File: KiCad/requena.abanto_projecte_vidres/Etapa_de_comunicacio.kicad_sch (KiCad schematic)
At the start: 13 parts, among them J1 DE9_Pins, J2 DE9_Pins, U1 MAX232, U3 TJA1051TK-3

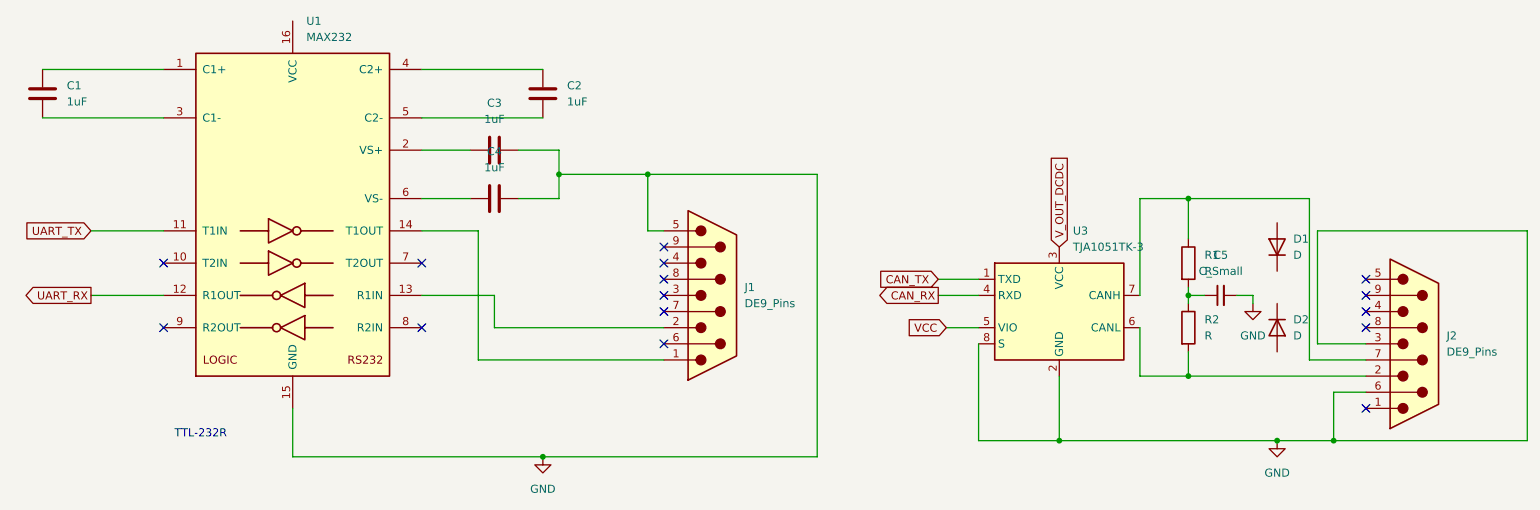
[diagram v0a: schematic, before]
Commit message: arreglos :)
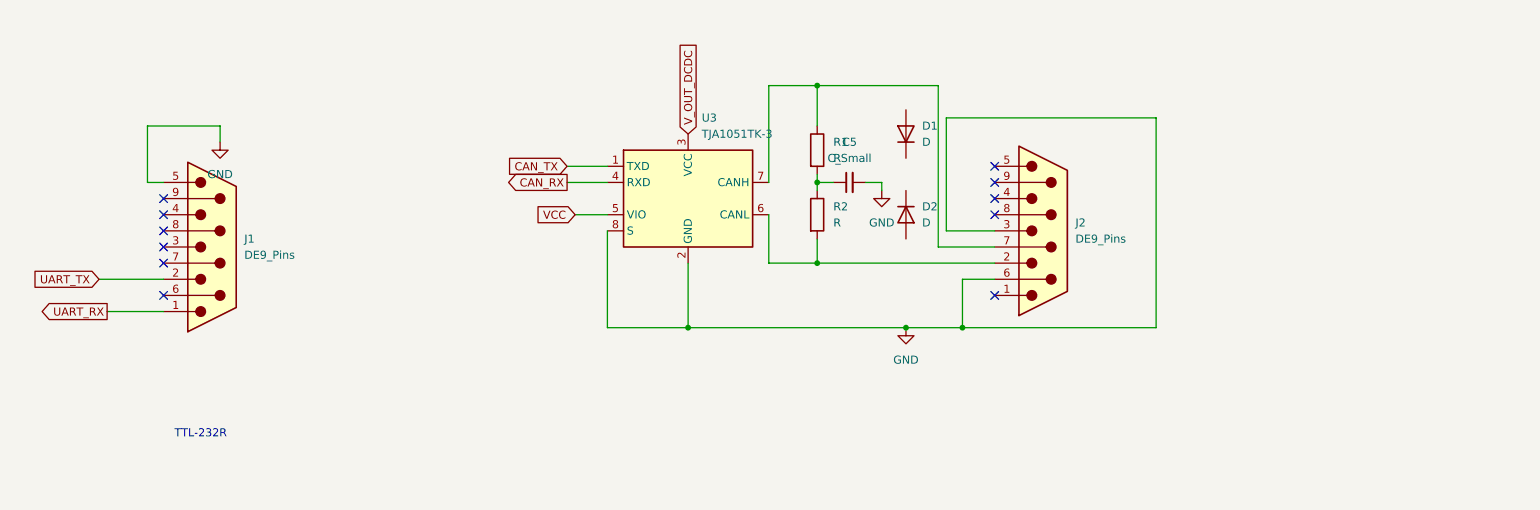
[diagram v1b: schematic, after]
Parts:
- removed C1, C2, C3, C4: 1uF, symbol Device:C
- removed U1: MAX232, symbol Interface_UART:MAX232
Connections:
- net UART_RX: now also J1.1
- net UART_TX: now also J1.2
- no-connect marks 15 -> 11
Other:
- moved on the sheet: C5, D1, D2, J1, J2, R1, R2, U3
